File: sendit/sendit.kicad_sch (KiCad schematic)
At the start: 7 parts, among them J1 Conn_01x02

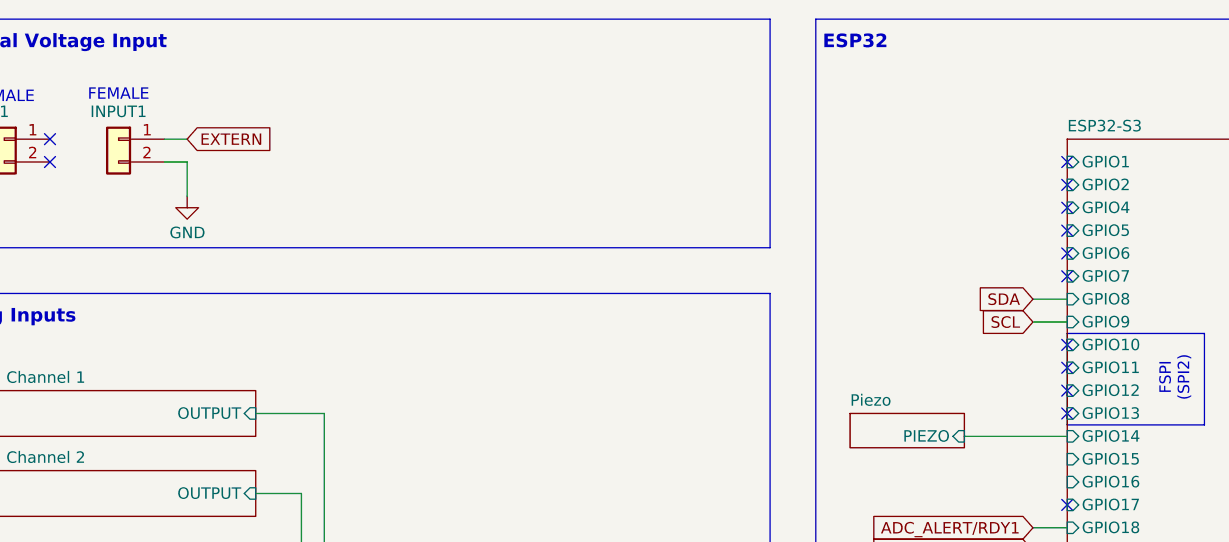
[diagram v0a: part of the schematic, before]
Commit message: more work on rev c board schematic
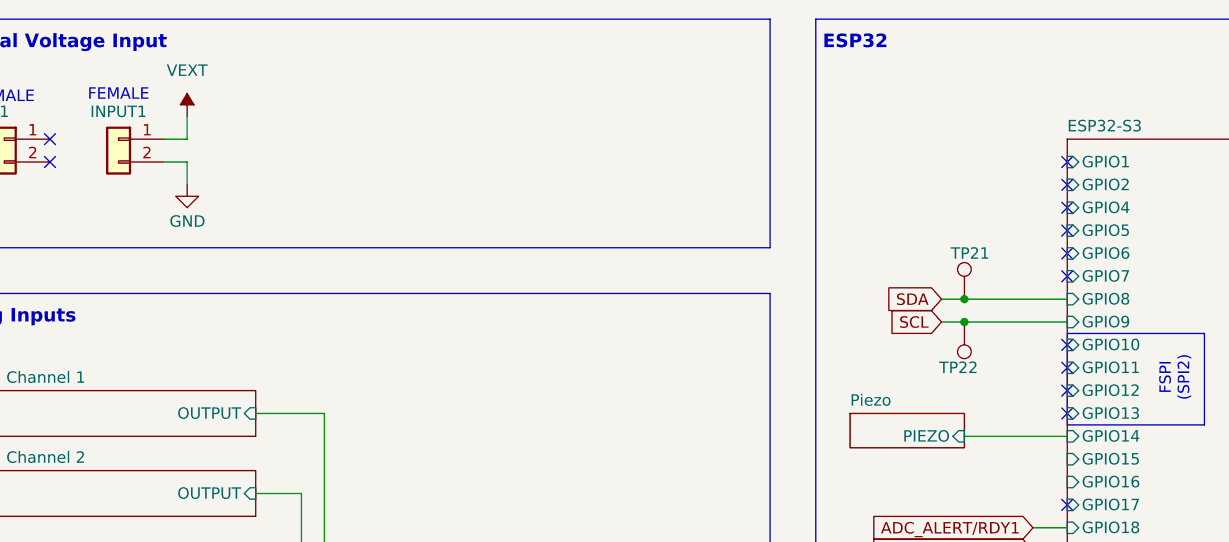
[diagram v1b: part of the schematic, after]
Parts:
- added TP21, TP22: ~, TestPoint:TestPoint_THTPad_D2.0mm_Drill1.0mm, symbol Connector:TestPoint
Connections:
- net SCL: now also TP22.1
- net SDA: now also TP21.1
- net EXTERN renamed VEXT
